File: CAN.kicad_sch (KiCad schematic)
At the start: 6 parts, among them IC1 ISO1050DUBR, IC2 ISO1050DUBR

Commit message: Layout updates
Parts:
- IC1, IC2: symbol MA_General:ISO1050DUBR -> MAG_CAN_Transceivers:ISO1050DUBR
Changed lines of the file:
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@@
     (pin "1")
   )
-  (symbol (lib_id "MA_General:ISO1050DUBR") (at 134.62 68.58 0) (unit 1)
+  (symbol (lib_id "MAG_CAN_Transceivers:ISO1050DUBR") (at 134.62 68.58 0) (unit 1)
     (in_bom yes) (on_board yes) (fields_autoplaced)
     (property "Reference" "IC1" (id 0) (at 148.59 60.96 0))
@@
     (pin "2")
   )
-  (symbol (lib_id "MA_General:ISO1050DUBR") (at 134.62 115.57 0) (unit 1)
+  (symbol (lib_id "MAG_CAN_Transceivers:ISO1050DUBR") (at 134.62 115.57 0) (unit 1)
     (in_bom yes) (on_board yes) (fields_autoplaced)
     (property "Reference" "IC2" (id 0) (at 148.59 107.95 0))

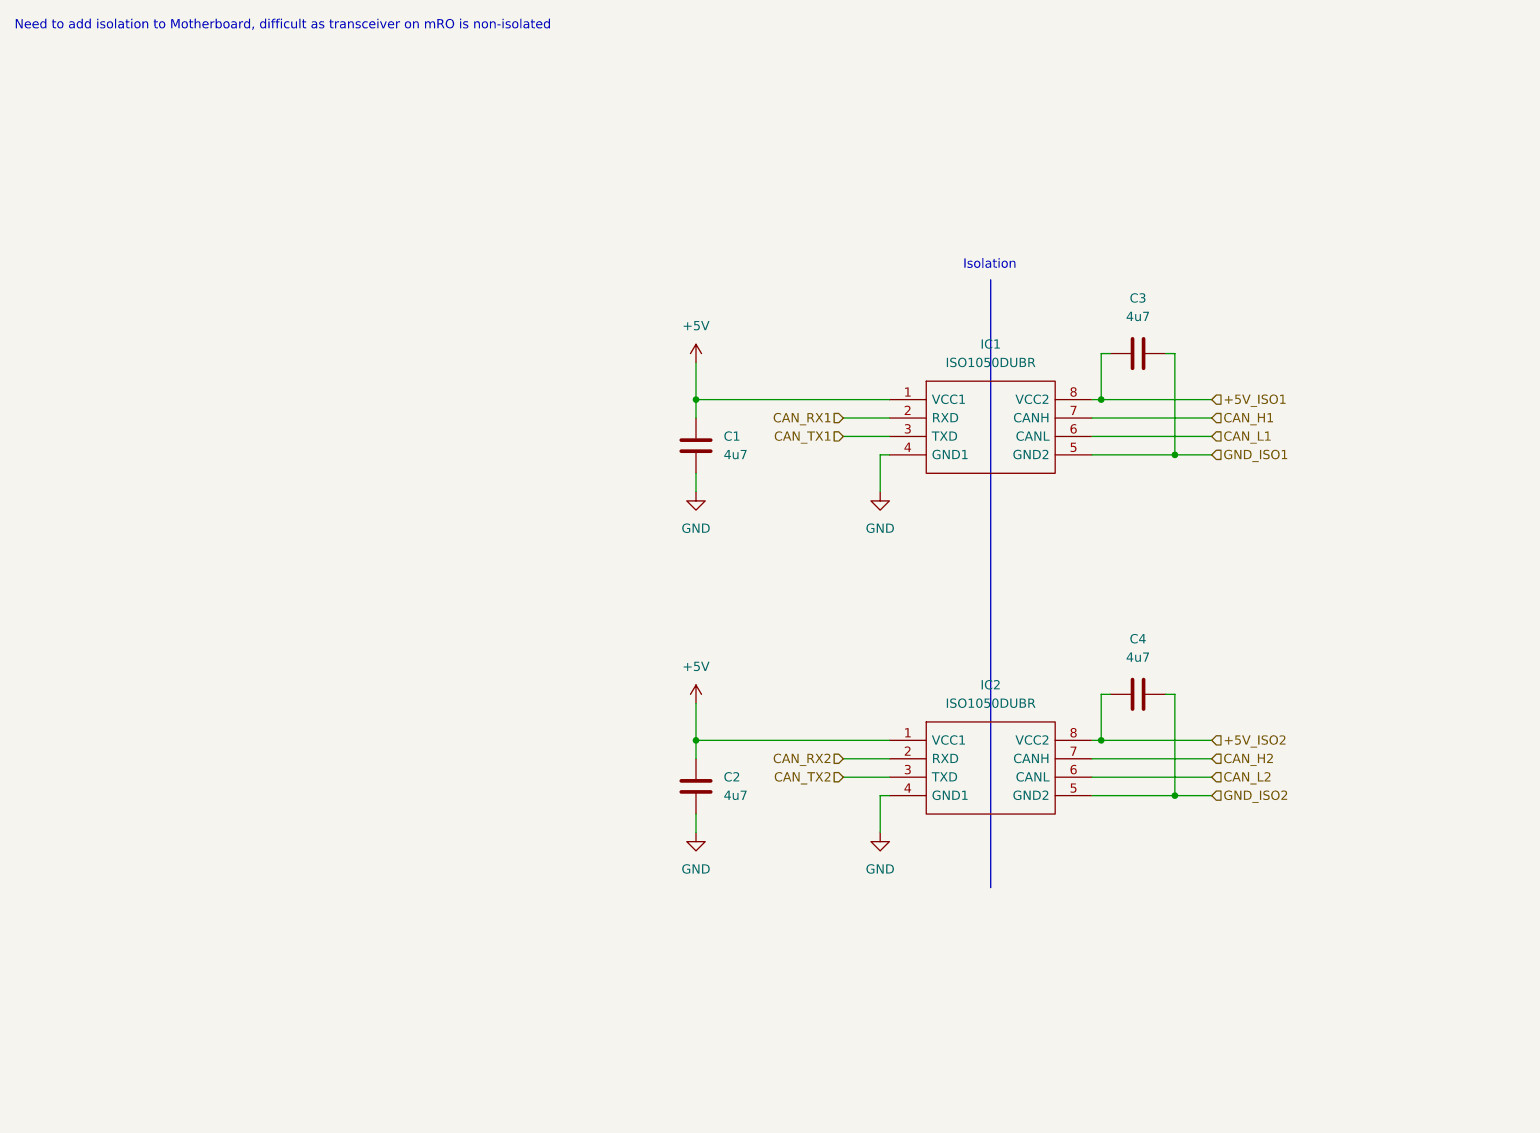
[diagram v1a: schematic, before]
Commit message: Updates for review
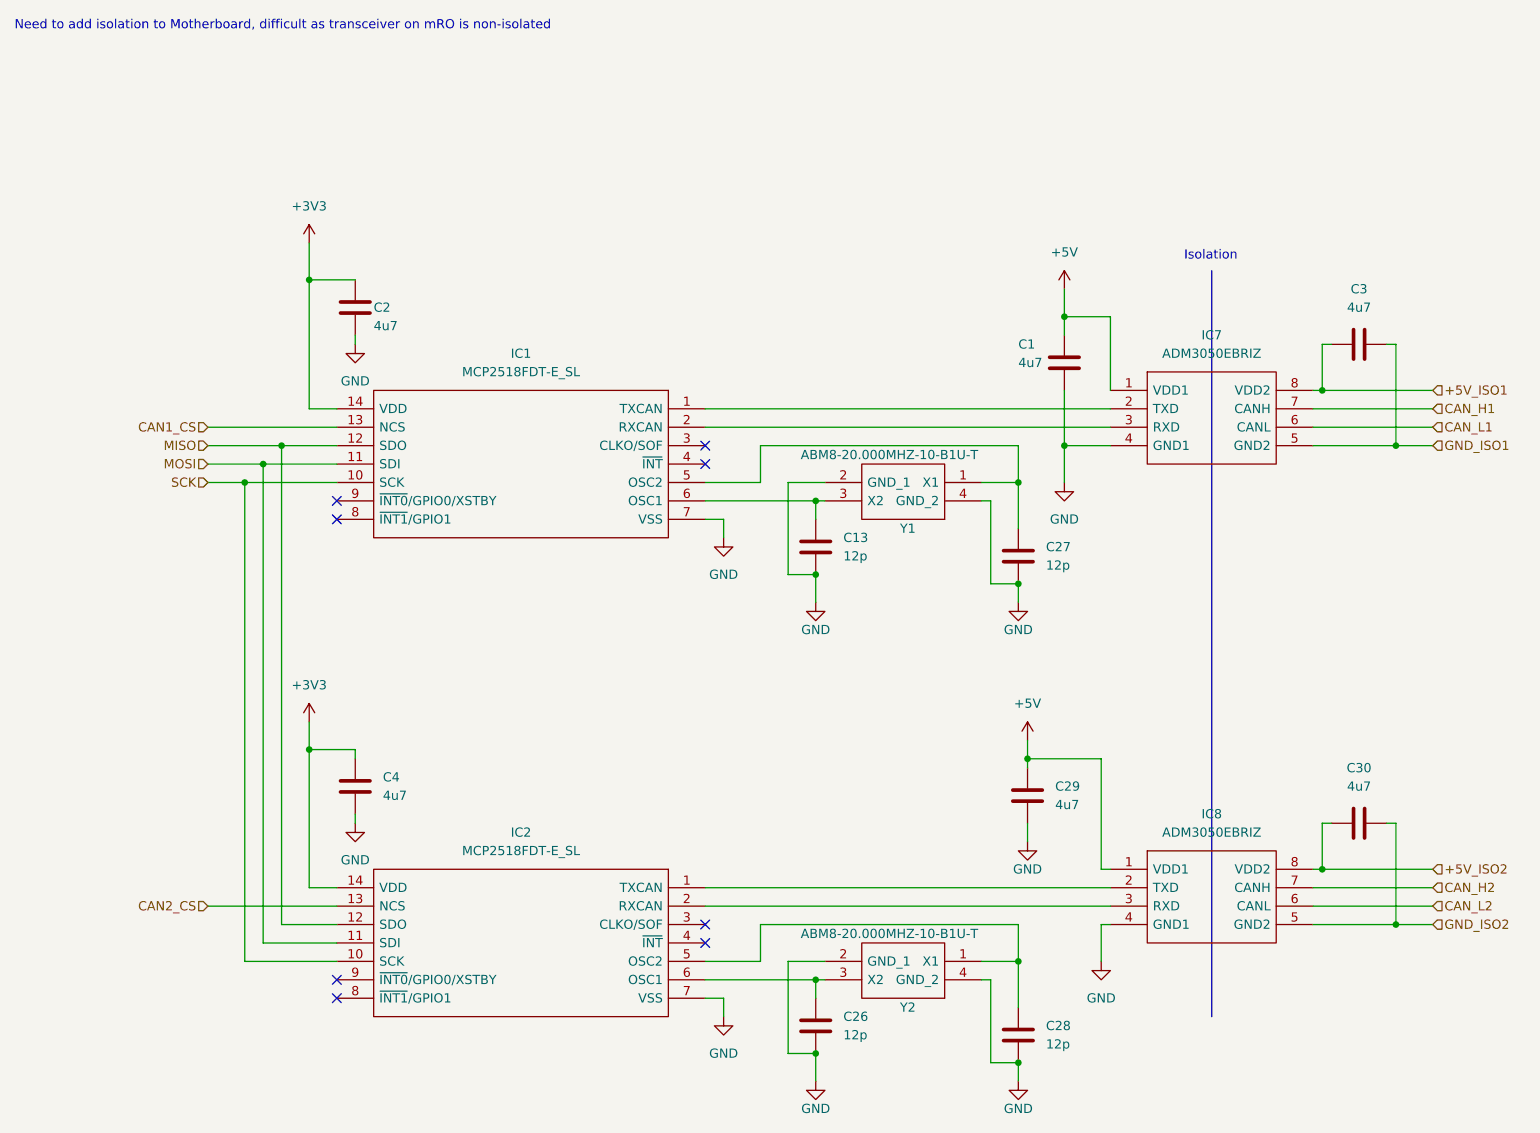
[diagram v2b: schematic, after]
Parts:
- removed IC1, IC2: ISO1050DUBR, SOP254P1040X485-8N, symbol MAG_CAN_Transceivers:ISO1050DUBR
- added C13, C26, C27, C28: 12p, Capacitor_SMD:C_0603_1608Metric, symbol Device:C
- added C29, C30: 4u7, Capacitor_SMD:C_0603_1608Metric, symbol Device:C
- added IC1, IC2: MCP2518FDT-E_SL, SOIC127P600X175-14N, symbol MAG_CAN_Transceivers:MCP2518FDT-E_SL
- added IC7, IC8: ADM3050EBRIZ, SOIC127P1031X265-8N, symbol MAG_CAN_Transceivers:ADM3050EBRIZ
- added Y1, Y2: ABM8-20.000MHZ-10-B1U-T, ABM810000MHZ12D2W, symbol MAG_Crystals:ABM8-20.000MHZ-10-B1U-T
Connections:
- net +5V: now also C29.1, IC7.1 (VDD1), IC8.1 (VDD1); no longer C2.1
- net +5V_ISO1: now also IC7.8 (VDD2)
- net +5V_ISO2: now also C30.1, IC8.8 (VDD2); no longer C4.1
- net CAN_H1: now also IC7.7 (CANH)
- net CAN_H2: now also IC8.7 (CANH)
- net CAN_L1: now also IC7.6 (CANL)
- net CAN_L2: now also IC8.6 (CANL)
- net GND: now also C4.2, C13.2, C26.2, C27.2, C28.2, C29.2, IC1.7 (VSS), IC2.7 (VSS), IC7.4 (GND1), IC8.4 (GND1), Y1.2 (GND_1), Y1.4 (GND_2), Y2.2 (GND_1), Y2.4 (GND_2)
- net GND_ISO1: now also IC7.5 (GND2)
- net GND_ISO2: now also C30.2, IC8.5 (GND2); no longer C4.2
- new net: IC1.1 (TXCAN), IC7.2 (TXD)
- new net: IC1.2 (RXCAN), IC7.3 (RXD)
- new net: C27.1, IC1.5 (OSC2), Y1.1 (X1)
- new net: C13.1, IC1.6 (OSC1), Y1.3 (X2)
- new net: IC2.1 (TXCAN), IC8.2 (TXD)
- new net: IC2.2 (RXCAN), IC8.3 (RXD)
- new net: C28.1, IC2.5 (OSC2), Y2.1 (X1)
- new net: C26.1, IC2.6 (OSC1), Y2.3 (X2)
- new net +3V3: C2.1, C4.1, IC1.14 (VDD), IC2.14 (VDD)
- new net CAN1_CS: IC1.13 (NCS)
- new net CAN2_CS: IC2.13 (NCS)
- new net MISO: IC1.12 (SDO), IC2.12 (SDO)
- new net MOSI: IC1.11 (SDI), IC2.11 (SDI)
- new net SCK: IC1.10 (SCK), IC2.10 (SCK)
- no-connect marks 0 -> 8
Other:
- moved on the sheet: C1, C3
